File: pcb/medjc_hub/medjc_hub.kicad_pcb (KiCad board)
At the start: 2 copper layers, 99 x 56 mm, 45 parts, among them J1 MJ-180P, J2 Conn_01x05_Socket, J3 Conn_01x05_Socket, J4 Conn_01x05_Socket, J5 Conn_01x02_Pin, U1 ESP32-C3_SUPERMINI, U2 BA033CC0T, U6 NJM2747D, U7 MCP3208-CI_P

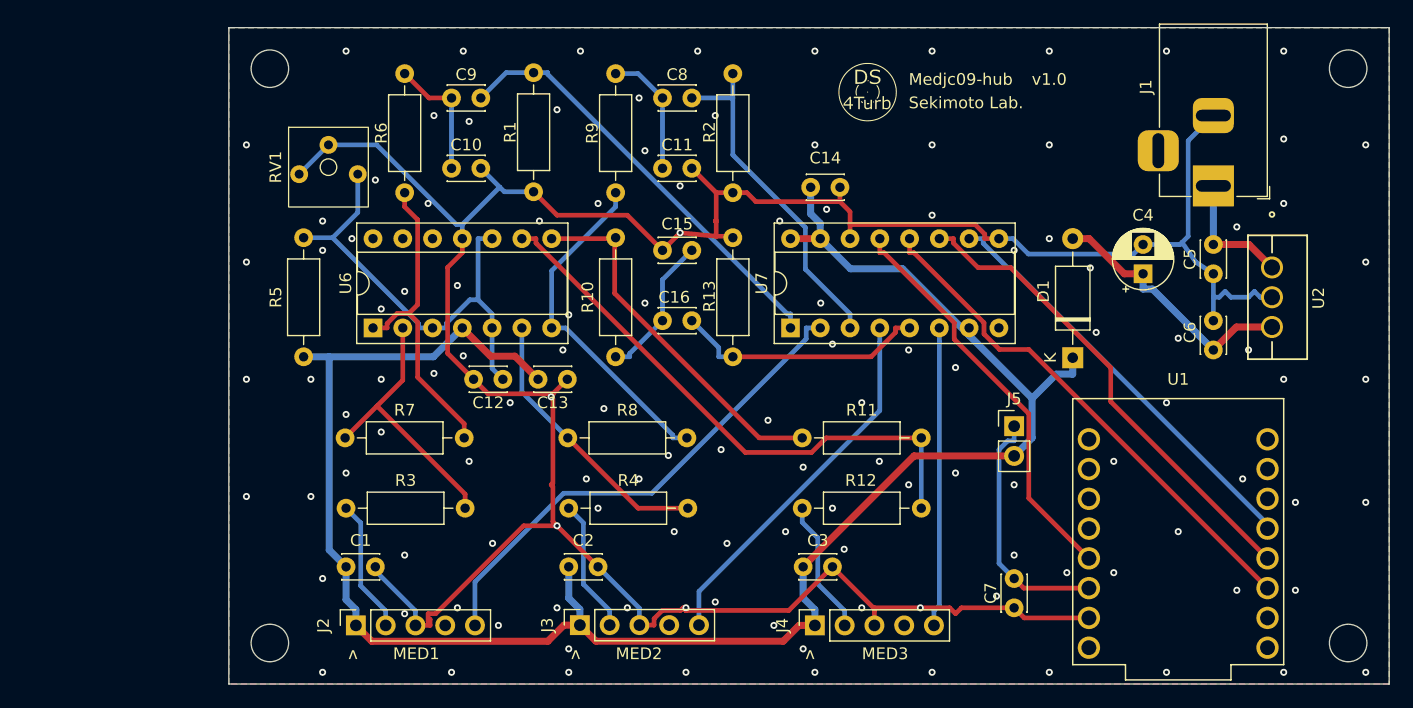
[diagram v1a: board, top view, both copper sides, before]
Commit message: 🍱 update: pcb v2
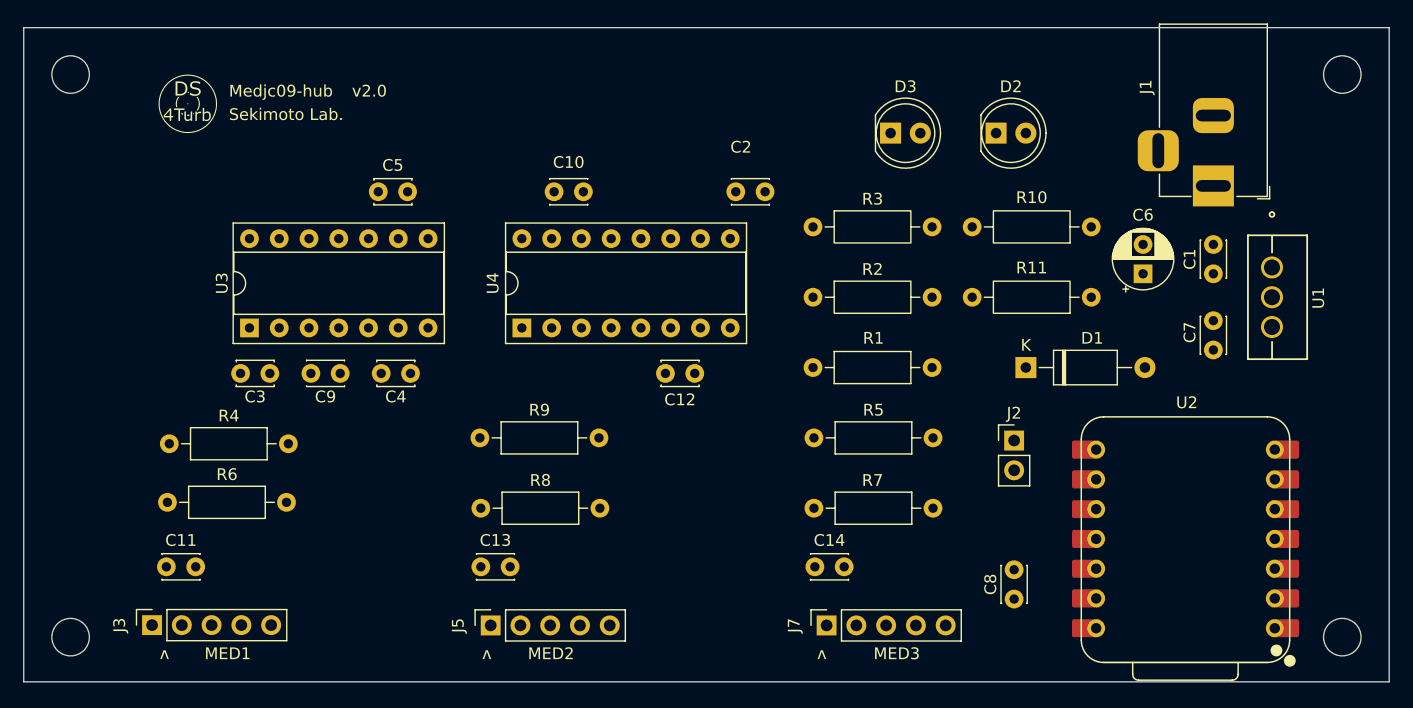
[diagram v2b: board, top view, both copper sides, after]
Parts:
- removed the C10 at (86.5, 82.0)
- removed the C11 at (102.0, 82.0)
- removed the C13 at (91.4, 100.0)
- removed C15: 1μF, Capacitor_THT:C_Disc_D3.0mm_W2.0mm_P2.50mm
- removed C16: 0.47μF, Capacitor_THT:C_Disc_D3.0mm_W2.0mm_P2.50mm
- removed the C8 at (104.5, 76.0)
- removed R13: 33kΩ, Resistor_THT:R_Axial_DIN0207_L6.3mm_D2.5mm_P10.16mm_Horizontal
- removed the R5 at (71.4, 98.1)
- removed the R6 at (80.0, 73.9)
- removed the R9 at (98.0, 73.9)
- removed RV1: 5kΩ, GF063:GF063P
- removed the U1 at (146.0, 113.0)
- added C12: 0.1μF, Capacitor_THT:C_Disc_D3.0mm_W2.0mm_P2.50mm, F.Cu at (104.8, 99.5)
- added C3: 0.1μF, Capacitor_THT:C_Disc_D3.0mm_W2.0mm_P2.50mm, F.Cu at (68.5, 99.5)
- added C4: 0.1μF, Capacitor_THT:C_Disc_D3.0mm_W2.0mm_P2.50mm, F.Cu at (78.0, 99.5)
- added C5: 0.1μF, Capacitor_THT:C_Disc_D3.0mm_W2.0mm_P2.50mm, F.Cu at (77.8, 84.0)
- added D2: LED, LED_THT:LED_D5.0mm, F.Cu at (130.5, 79.0)
- added D3: LED, LED_THT:LED_D5.0mm, F.Cu at (121.5, 79.0)
- added R11: 200Ω, Resistor_THT:R_Axial_DIN0207_L6.3mm_D2.5mm_P10.16mm_Horizontal, F.Cu at (138.6, 93.0)
- added R3: 5kΩ, Resistor_THT:R_Axial_DIN0207_L6.3mm_D2.5mm_P10.16mm_Horizontal, F.Cu at (114.8, 87.0)
- added U2: XIAO-ESP32-S3-DIP, Seeed Studio XIAO Series Library:XIAO-ESP32S3-DIP, F.Cu at (146.6, 113.6)
- C9: value 0.47μF -> 0.1μF
- R1, R2: value 33kΩ -> 10kΩ
- moved REF3 109.0 mm to (51.5, 74.0)
- moved REF4 109.0 mm to (51.5, 122.0)
- moved REF1 91.5 mm to (160.0, 74.0)
- moved REF2 91.5 mm to (160.0, 122.0)
- moved G*** 58.0 mm to (61.5, 76.5)
- moved R10 40.6 mm to (138.6, 87.0), turned to 180 degrees
- moved R1 37.2 mm to (125.0, 99.0), turned to 180 degrees
- moved C9 26.4 mm to (74.5, 99.5)
- moved C2 25.5 mm to (108.2, 84.0), turned to 0 degrees
- moved U4 22.9 mm to (90.0, 95.6)
- moved C10 21.9 mm to (92.8, 84.0)
- moved R2 20.3 mm to (114.8, 93.0), turned to 0 degrees
- moved J3 17.4 mm to (58.5, 121.0)
- moved C11 15.3 mm to (59.7, 116.0)
- moved R6 15.2 mm to (59.8, 110.5)
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- renumbered C5 to C1, C14 to C10, C1 to C11, C2 to C13, C3 to C14, C12 to C2, C4 to C6, C6 to C7, C7 to C8, J5 to J2, J2 to J3, J3 to J5, J4 to J7, R7 to R4, R11 to R5, R3 to R6, R12 to R7, R4 to R8, R8 to R9, U2 to U1, U6 to U3, U7 to U4
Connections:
- C2 pad 1: Net-(U6-+IN_A) -> IN_AMP_A
- C9 pad 1: FME1 -> +3V3
- C9 pad 2: Net-(C10-Pad2) -> GND
- J3 pad 4: unconnected-(J2-Pin_4-Pad4) -> Net-(J3-Pin_4)
- J5 pad 4: unconnected-(J3-Pin_4-Pad4) -> Net-(J3-Pin_4)
- J7 pad 4: unconnected-(J4-Pin_4-Pad4) -> Net-(J3-Pin_4)
- R1 pad 1: GND -> +3V3
- R1 pad 2: FME1 -> IN_AMP_A
- R10 pad 1: Net-(U6-OUT_C) -> POWER_LED
- R2 pad 1: FME2 -> IN_AMP_A
- R4 pad 2: Net-(U6-OUT_A) -> FME1
- R5 pad 1: Net-(U6-OUT_C) -> FME3
- R9 pad 2: Net-(U6-OUT_B) -> FME2
- U3 pad 1: Net-(U6-OUT_A) -> FME1
- U3 pad 10: Net-(U6-+IN_A) -> IN_AMP_A
- U3 pad 3: Net-(U6-+IN_A) -> IN_AMP_A
- U3 pad 5: Net-(U6-+IN_A) -> IN_AMP_A
- U3 pad 7: Net-(U6-OUT_B) -> FME2
- U3 pad 8: Net-(U6-OUT_C) -> FME3
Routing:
- net GND: track 240.1 -> 0.00 mm, vias 124 -> 0
- net +3V3: track 163.7 -> 0.00 mm
- net Net-(U3--IN_C): track 48.4 -> 0.00 mm
- net MISO: track 44.2 -> 0.00 mm
- net SME1: track 42.7 -> 0.00 mm
- net MOSI: track 41.2 -> 0.00 mm
- net Net-(U6-+IN_A): track 39.9 -> 0.00 mm
- net FME1: track 37.1 -> 0.00 mm
- net SS: track 36.2 -> 0.00 mm
- net SCK: track 34.9 -> 0.00 mm
- net SME2: track 31.7 -> 0.00 mm
- net Net-(U6-OUT_C): track 31.3 -> 0.00 mm
- net Net-(U6-OUT_B): track 29.4 -> 0.00 mm
- net FME2: track 29.3 -> 0.00 mm
- net Net-(U6-OUT_A): track 27.4 -> 0.00 mm
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- removed copper zone on B.Cu, net GND
- removed copper zone on F.Cu, net GND
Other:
- board size 99 x 56 mm -> 116.5 x 55.8 mm
- board text added: "K"
- board text added: "v2.0"
- board text removed: "v1.0"
